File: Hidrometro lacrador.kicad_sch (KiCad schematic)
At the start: 2 parts, among them J1 Screw_Terminal_01x03, U1 ESP32-WROOM-V1

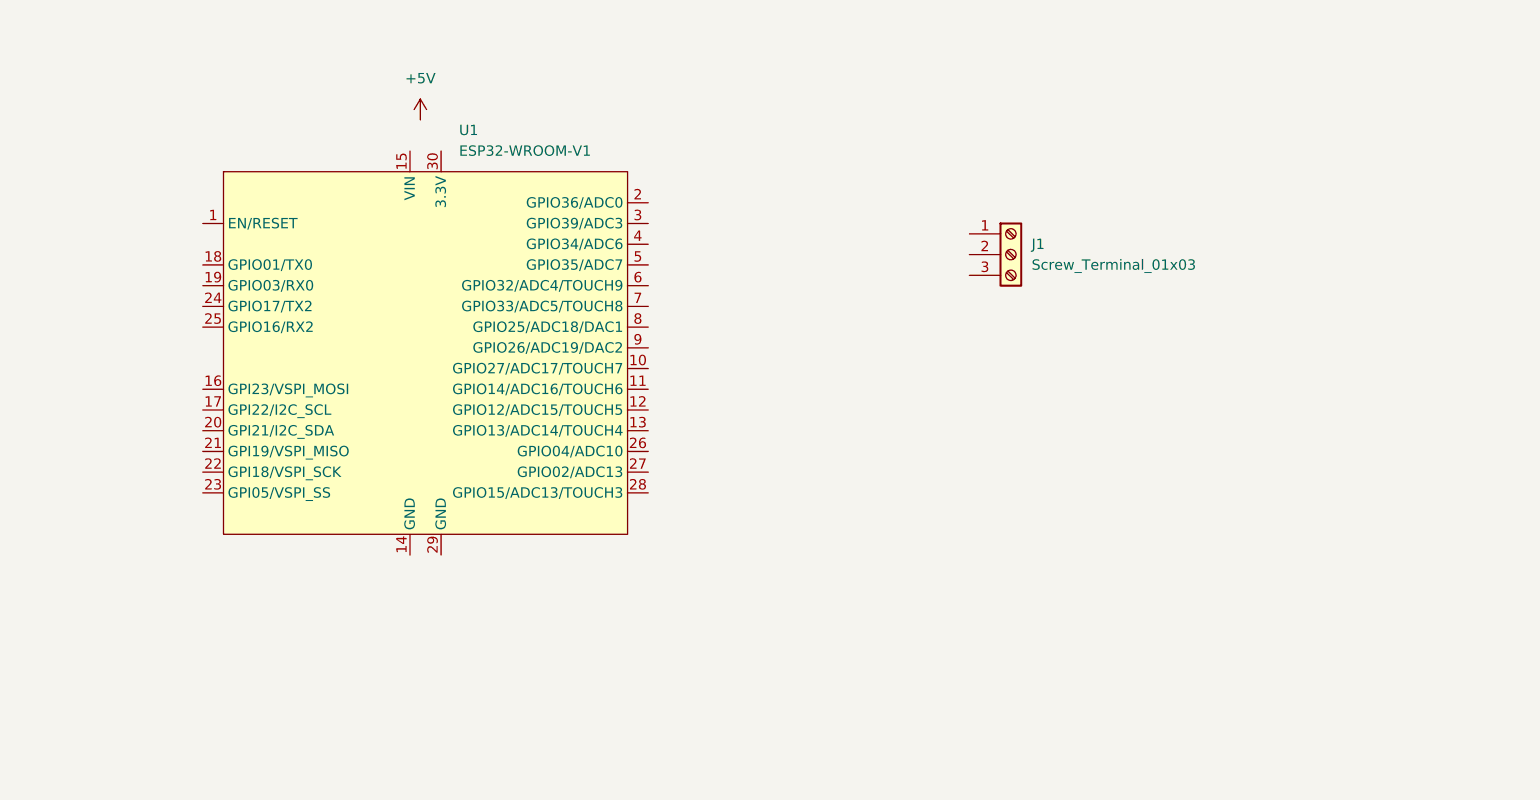
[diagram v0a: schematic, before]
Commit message: Disposição dos componentes na PCB
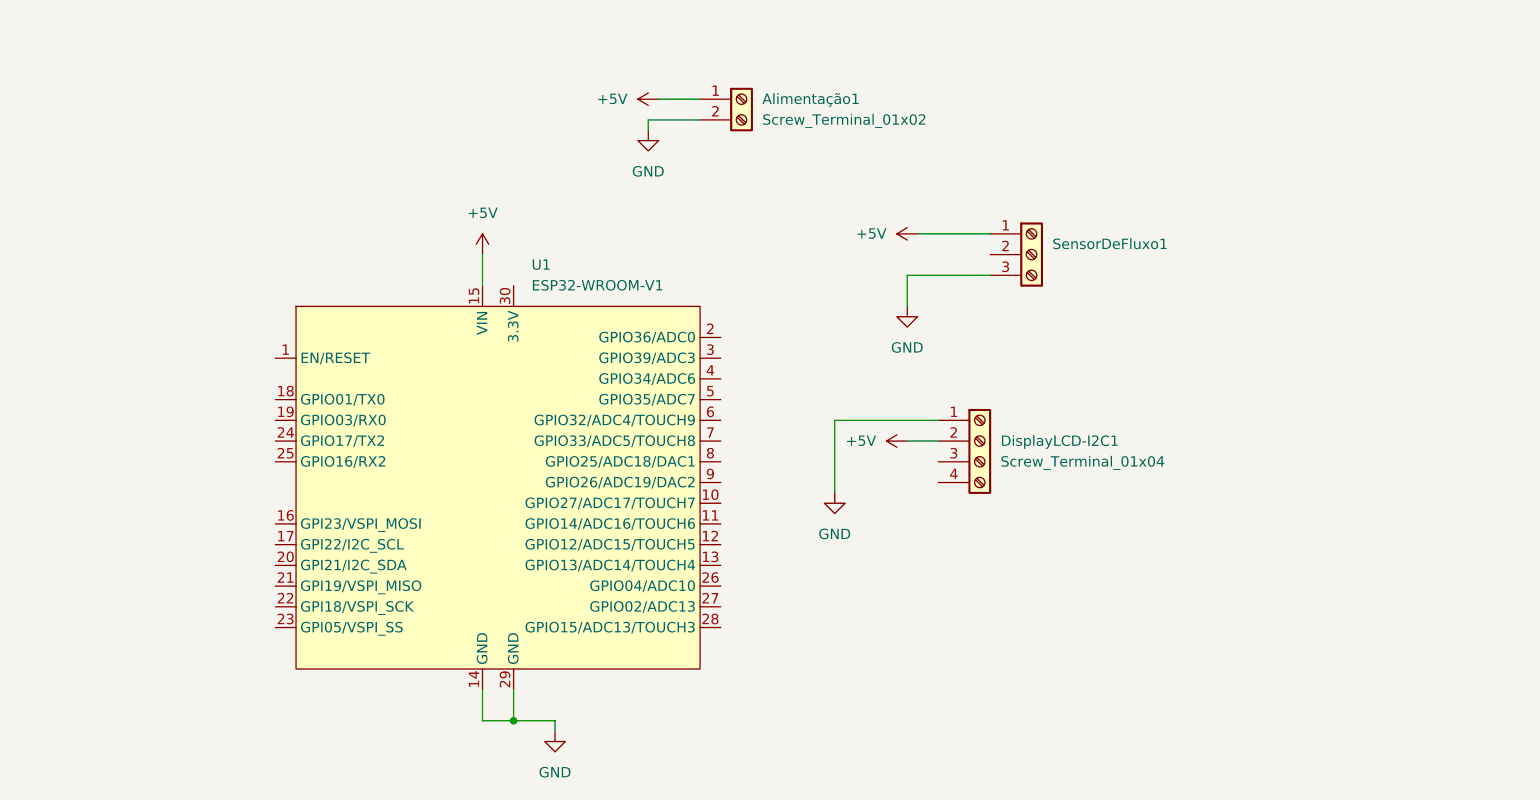
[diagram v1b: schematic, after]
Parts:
- added Alimentação1: Screw_Terminal_01x02, TerminalBlock:TerminalBlock_Altech_AK300-2_P5.00mm, symbol Connector:Screw_Terminal_01x02
- added DisplayLCD-I2C1: Screw_Terminal_01x04, TerminalBlock:TerminalBlock_Altech_AK300-4_P5.00mm, symbol Connector:Screw_Terminal_01x04
- SensorDeFluxo1: renamed from J1; footprint (none) -> TerminalBlock:TerminalBlock_Altech_AK300-3_P5.00mm
- U1: footprint (none) -> ESP:ESP32-WROOM
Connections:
- net +5V: now also SensorDeFluxo1.1 (Pin_1), U1.15 (VIN), Alimentação1.1 (Pin_1), DisplayLCD-I2C1.2 (Pin_2)
- net GND: now reaches U1.14 (GND)
- net GND: now also SensorDeFluxo1.3 (Pin_3), U1.29 (GND), Alimentação1.2 (Pin_2), DisplayLCD-I2C1.1 (Pin_1)
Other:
- moved on the sheet: SensorDeFluxo1, U1

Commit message: Finalização do circuito e da PCB
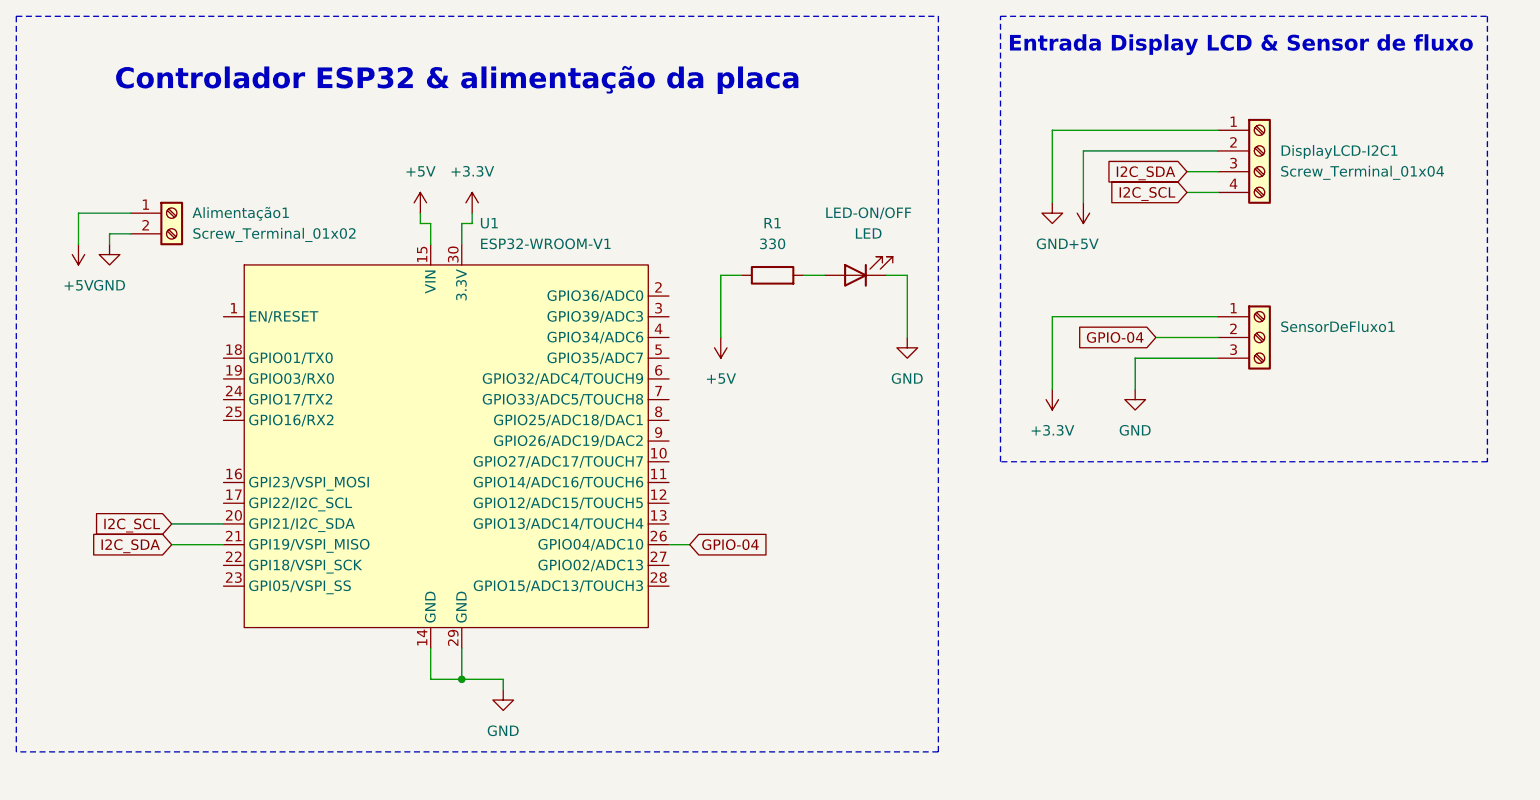
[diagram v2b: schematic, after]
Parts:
- added LED-ON/OFF: LED, TerminalBlock:TerminalBlock_Altech_AK300-2_P5.00mm, symbol Device:LED
- added R1: 330, Resistor_THT:R_Axial_DIN0414_L11.9mm_D4.5mm_P20.32mm_Horizontal, symbol Device:R
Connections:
- net +5V: now also R1.1; no longer SensorDeFluxo1.1 (Pin_1)
- net GND: now also LED-ON/OFF.1 (K)
- net I2C_SCL: now reaches U1.20 (GPI21/I2C_SDA)
- net I2C_SCL: now also DisplayLCD-I2C1.4 (Pin_4)
- net I2C_SDA: now reaches U1.21 (GPI19/VSPI_MISO)
- net I2C_SDA: now also DisplayLCD-I2C1.3 (Pin_3)
- net GPIO-04: now reaches U1.26 (GPIO04/ADC10)
- net GPIO-04: now also SensorDeFluxo1.2 (Pin_2)
- net +3.3V: now reaches U1.30 (3.3V)
- net +3.3V: now also SensorDeFluxo1.1 (Pin_1)
- new net: LED-ON/OFF.2 (A), R1.2
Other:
- note added: "Controlador ESP32 & alimentação da placa"
- note added: "Entrada Display LCD & Sensor de fluxo"
- moved on the sheet: Alimentação1, DisplayLCD-I2C1, SensorDeFluxo1, U1

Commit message: mudança das portas do display LCD
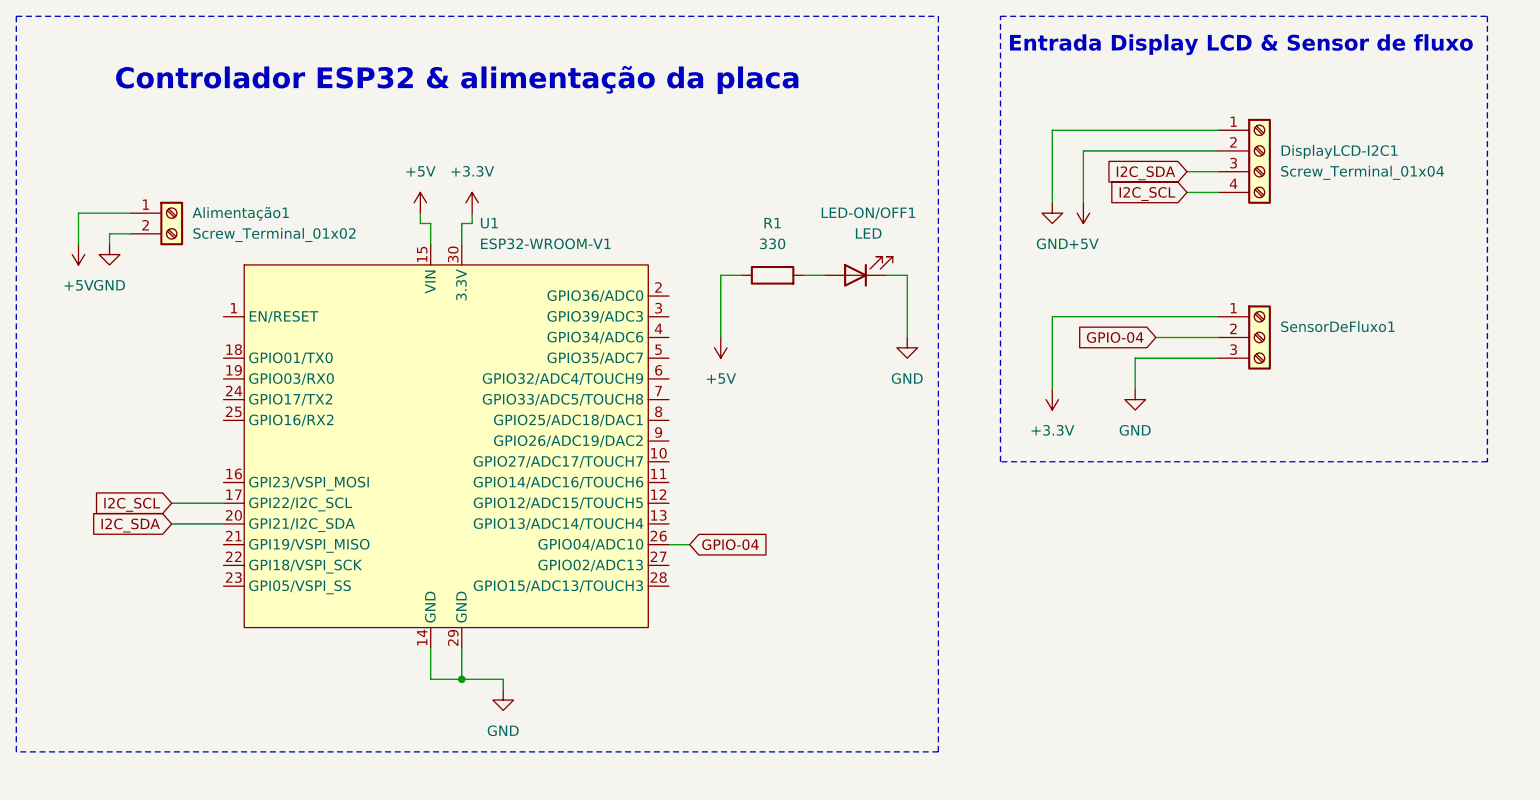
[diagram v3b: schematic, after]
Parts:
- renumbered LED-ON/OFF to LED-ON/OFF1
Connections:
- net I2C_SCL: now also U1.17 (GPI22/I2C_SCL); no longer U1.20 (GPI21/I2C_SDA)
- net I2C_SDA: now also U1.20 (GPI21/I2C_SDA); no longer U1.21 (GPI19/VSPI_MISO)
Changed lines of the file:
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@@
-	(wire
-		(pts
-			(xy 73.66 80.01) (xy 80.01 80.01)
-		)
-		(stroke
-			(width 0)
-			(type default)
-		)
-	)
 	(wire
 		(pts
@@
 	(wire
 		(pts
+			(xy 109.22 96.52) (xy 109.22 92.71)
+		)
+		(stroke
+			(width 0)
+			(type default)
+		)
+	)
+	(wire
+		(pts
+			(xy 151.13 46.99) (xy 153.67 46.99)
+		)
+		(stroke
+			(width 0)
+			(type default)
+		)
+	)
+	(wire
+		(pts
+			(xy 66.04 41.91) (xy 68.58 41.91)
+		)
+		(stroke
+			(width 0)
+			(type default)
+		)
+	)
+	(wire
+		(pts
+			(xy 181.61 29.21) (xy 201.93 29.21)
+		)
+		(stroke
+			(width 0)
+			(type default)
+		)
+	)
+	(wire
+		(pts
+			(xy 134.62 80.01) (xy 137.16 80.01)
+		)
+		(stroke
+			(width 0)
+			(type default)
+		)
+	)
+	(wire
+		(pts
+			(xy 163.83 46.99) (xy 163.83 54.61)
+		)
+		(stroke
+			(width 0)
+			(type default)
+		)
+	)
+	(wire
+		(pts
+			(xy 191.77 57.15) (xy 201.93 57.15)
+		)
+		(stroke
+			(width 0)
+			(type default)
+		)
+	)
+	(wire
+		(pts
+			(xy 185.42 38.1) (xy 185.42 31.75)
+		)
+		(stroke
+			(width 0)
+			(type default)
+		)
+	)
+	(wire
+		(pts
+			(xy 105.41 96.52) (xy 105.41 92.71)
+		)
+		(stroke
+			(width 0)
+			(type default)
+		)
+	)
+	(wire
+		(pts
+			(xy 66.04 43.18) (xy 66.04 41.91)
+		)
+		(stroke
+			(width 0)
+			(type default)
+		)
+	)
+	(wire
+		(pts
+			(xy 140.97 54.61) (xy 140.97 46.99)
+		)
+		(stroke
+			(width 0)
+			(type default)
+		)
+	)
+	(wire
+		(pts
 			(xy 73.66 77.47) (xy 80.01 77.47)
 		)
@@
 	(wire
 		(pts
-			(xy 109.22 96.52) (xy 109.22 92.71)
-		)
-		(stroke
-			(width 0)
-			(type default)
-		)
-	)
-	(wire
-		(pts
-			(xy 151.13 46.99) (xy 153.67 46.99)
-		)
-		(stroke
-			(width 0)
-			(type default)
-		)
-	)
-	(wire
-		(pts
-			(xy 66.04 41.91) (xy 68.58 41.91)
-		)
-		(stroke
-			(width 0)
-			(type default)
-		)
-	)
-	(wire
-		(pts
-			(xy 181.61 29.21) (xy 201.93 29.21)
-		)
-		(stroke
-			(width 0)
-			(type default)
-		)
-	)
-	(wire
-		(pts
-			(xy 134.62 80.01) (xy 137.16 80.01)
-		)
-		(stroke
-			(width 0)
-			(type default)
-		)
-	)
-	(wire
-		(pts
-			(xy 163.83 46.99) (xy 163.83 54.61)
-		)
-		(stroke
-			(width 0)
-			(type default)
-		)
-	)
-	(wire
-		(pts
-			(xy 191.77 57.15) (xy 201.93 57.15)
-		)
-		(stroke
-			(width 0)
-			(type default)
-		)
-	)
-	(wire
-		(pts
-			(xy 185.42 38.1) (xy 185.42 31.75)
-		)
-		(stroke
-			(width 0)
-			(type default)
-		)
-	)
-	(wire
-		(pts
-			(xy 105.41 96.52) (xy 105.41 92.71)
-		)
-		(stroke
-			(width 0)
-			(type default)
-		)
-	)
-	(wire
-		(pts
-			(xy 66.04 43.18) (xy 66.04 41.91)
-		)
-		(stroke
-			(width 0)
-			(type default)
-		)
-	)
-	(wire
-		(pts
-			(xy 140.97 54.61) (xy 140.97 46.99)
-		)
-		(stroke
-			(width 0)
-			(type default)
-		)
-	)
-	(wire
-		(pts
 			(xy 109.22 40.64) (xy 109.22 43.18)
 		)
@@
 		(pts
 			(xy 105.41 40.64) (xy 105.41 43.18)
+		)
+		(stroke
+			(width 0)
+			(type default)
+		)
+	)
+	(wire
+		(pts
+			(xy 73.66 74.93) (xy 80.01 74.93)
 		)
 		(stroke
@@
 	(global_label "I2C_SCL"
 		(shape input)
+		(at 73.66 74.93 180)
+		(fields_autoplaced yes)
+		(effects
+			(font
+				(size 1.27 1.27)
+			)
+			(justify right)
+		)
+		(property "Intersheetrefs" "${INTERSHEET_REFS}"
+			(at 63.1153 74.93 0)
+			(effects
+				(font
+					(size 1.27 1.27)
+				)
+				(justify right)
+				(hide yes)
+			)
+		)
+	)
+	(global_label "I2C_SCL"
+		(shape input)
+		(at 198.12 36.83 180)
+		(fields_autoplaced yes)
+		(effects
+			(font
+				(size 1.27 1.27)
+			)
+			(justify right)
+		)
+		(property "Intersheetrefs" "${INTERSHEET_REFS}"
+			(at 187.5753 36.83 0)
+			(effects
+				(font
+					(size 1.27 1.27)
+				)
+				(justify right)
+				(hide yes)
+			)
+		)
+	)
+	(global_label "GPIO-04"
+		(shape input)
+		(at 137.16 80.01 0)
+		(fields_autoplaced yes)
+		(effects
+			(font
+				(size 1.27 1.27)
+			)
+			(justify left)
+		)
+		(property "Intersheetrefs" "${INTERSHEET_REFS}"
+			(at 148.6119 80.01 0)
+			(effects
+				(font
+					(size 1.27 1.27)
+				)
+				(justify left)
+				(hide yes)
+			)
+		)
+	)
+	(global_label "GPIO-04"
+		(shape input)
+		(at 194.31 54.61 180)
+		(fields_autoplaced yes)
+		(effects
+			(font
+				(size 1.27 1.27)
+			)
+			(justify right)
+		)
+		(property "Intersheetrefs" "${INTERSHEET_REFS}"
+			(at 182.8581 54.61 0)
+			(effects
+				(font
+					(size 1.27 1.27)
+				)
+				(justify right)
+				(hide yes)
+			)
+		)
+	)
+	(global_label "I2C_SDA"
+		(shape input)
 		(at 73.66 77.47 180)
 		(fields_autoplaced yes)
@@
 		)
 		(property "Intersheetrefs" "${INTERSHEET_REFS}"
-			(at 63.1153 77.47 0)
-			(effects
-				(font
-					(size 1.27 1.27)
-				)
-				(justify right)
-				(hide yes)
-			)
-		)
-	)
-	(global_label "I2C_SCL"
-		(shape input)
-		(at 198.12 36.83 180)
-		(fields_autoplaced yes)
-		(effects
-			(font
-				(size 1.27 1.27)
-			)
-			(justify right)
-		)
-		(property "Intersheetrefs" "${INTERSHEET_REFS}"
-			(at 187.5753 36.83 0)
-			(effects
-				(font
-					(size 1.27 1.27)
-				)
-				(justify right)
-				(hide yes)
-			)
-		)
-	)
-	(global_label "GPIO-04"
-		(shape input)
-		(at 137.16 80.01 0)
-		(fields_autoplaced yes)
-		(effects
-			(font
-				(size 1.27 1.27)
-			)
-			(justify left)
-		)
-		(property "Intersheetrefs" "${INTERSHEET_REFS}"
-			(at 148.6119 80.01 0)
-			(effects
-				(font
-					(size 1.27 1.27)
-				)
-				(justify left)
-				(hide yes)
-			)
-		)
-	)
-	(global_label "GPIO-04"
-		(shape input)
-		(at 194.31 54.61 180)
-		(fields_autoplaced yes)
-		(effects
-			(font
-				(size 1.27 1.27)
-			)
-			(justify right)
-		)
-		(property "Intersheetrefs" "${INTERSHEET_REFS}"
-			(at 182.8581 54.61 0)
-			(effects
-				(font
-					(size 1.27 1.27)
-				)
-				(justify right)
-				(hide yes)
-			)
-		)
-	)
-	(global_label "I2C_SDA"
-		(shape input)
-		(at 73.66 80.01 180)
-		(fields_autoplaced yes)
-		(effects
-			(font
-				(size 1.27 1.27)
-			)
-			(justify right)
-		)
-		(property "Intersheetrefs" "${INTERSHEET_REFS}"
-			(at 63.0548 80.01 0)
+			(at 63.0548 77.47 0)
 			(effects
 				(font
@@
 		(dnp no)
 		(fields_autoplaced yes)
-		(property "Reference" "LED-ON/OFF"
+		(property "Reference" "LED-ON/OFF1"
 			(at 159.0675 39.37 0)
 			(effects
@@
 			(project "Hidrometro lacrador"
 				(path "/81a4609d-2271-43ec-aee9-d7a68edf5121"
-					(reference "LED-ON/OFF")
+					(reference "LED-ON/OFF1")
 					(unit 1)
 				)
